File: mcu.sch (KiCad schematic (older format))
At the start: 16 parts, among them SW1 SW_PUSH, U1 STM32F411RE_LQFP64, X1 32.768K, X2 8MHz

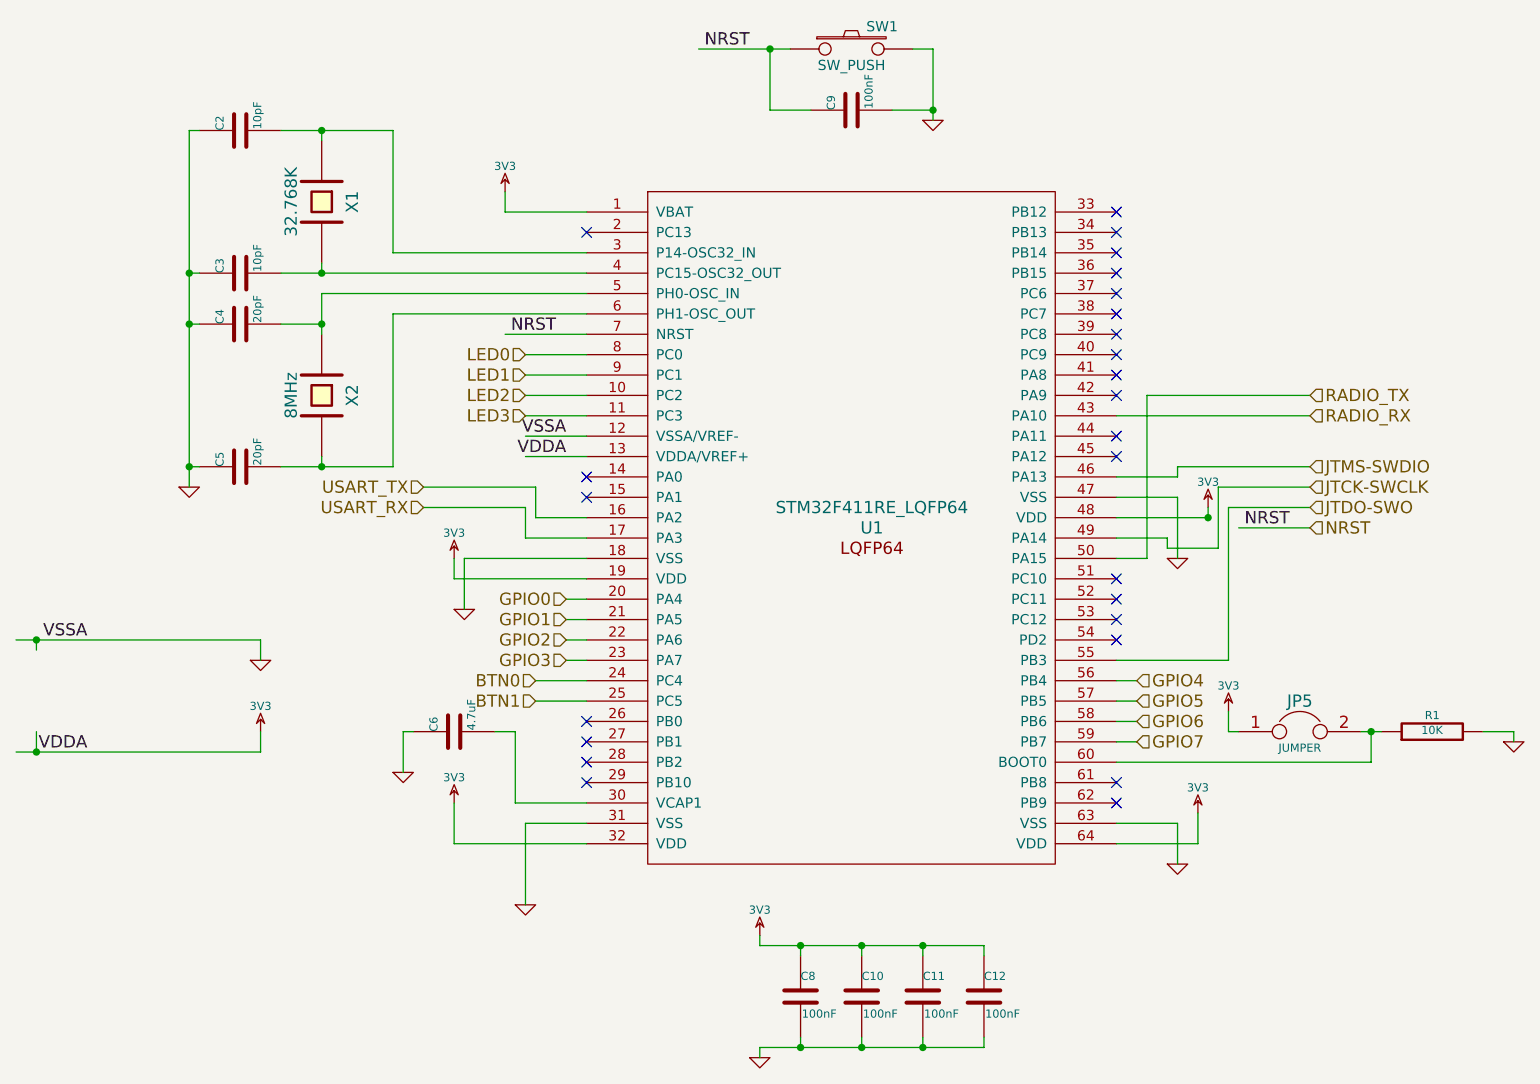
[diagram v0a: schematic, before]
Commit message: Made breakout board
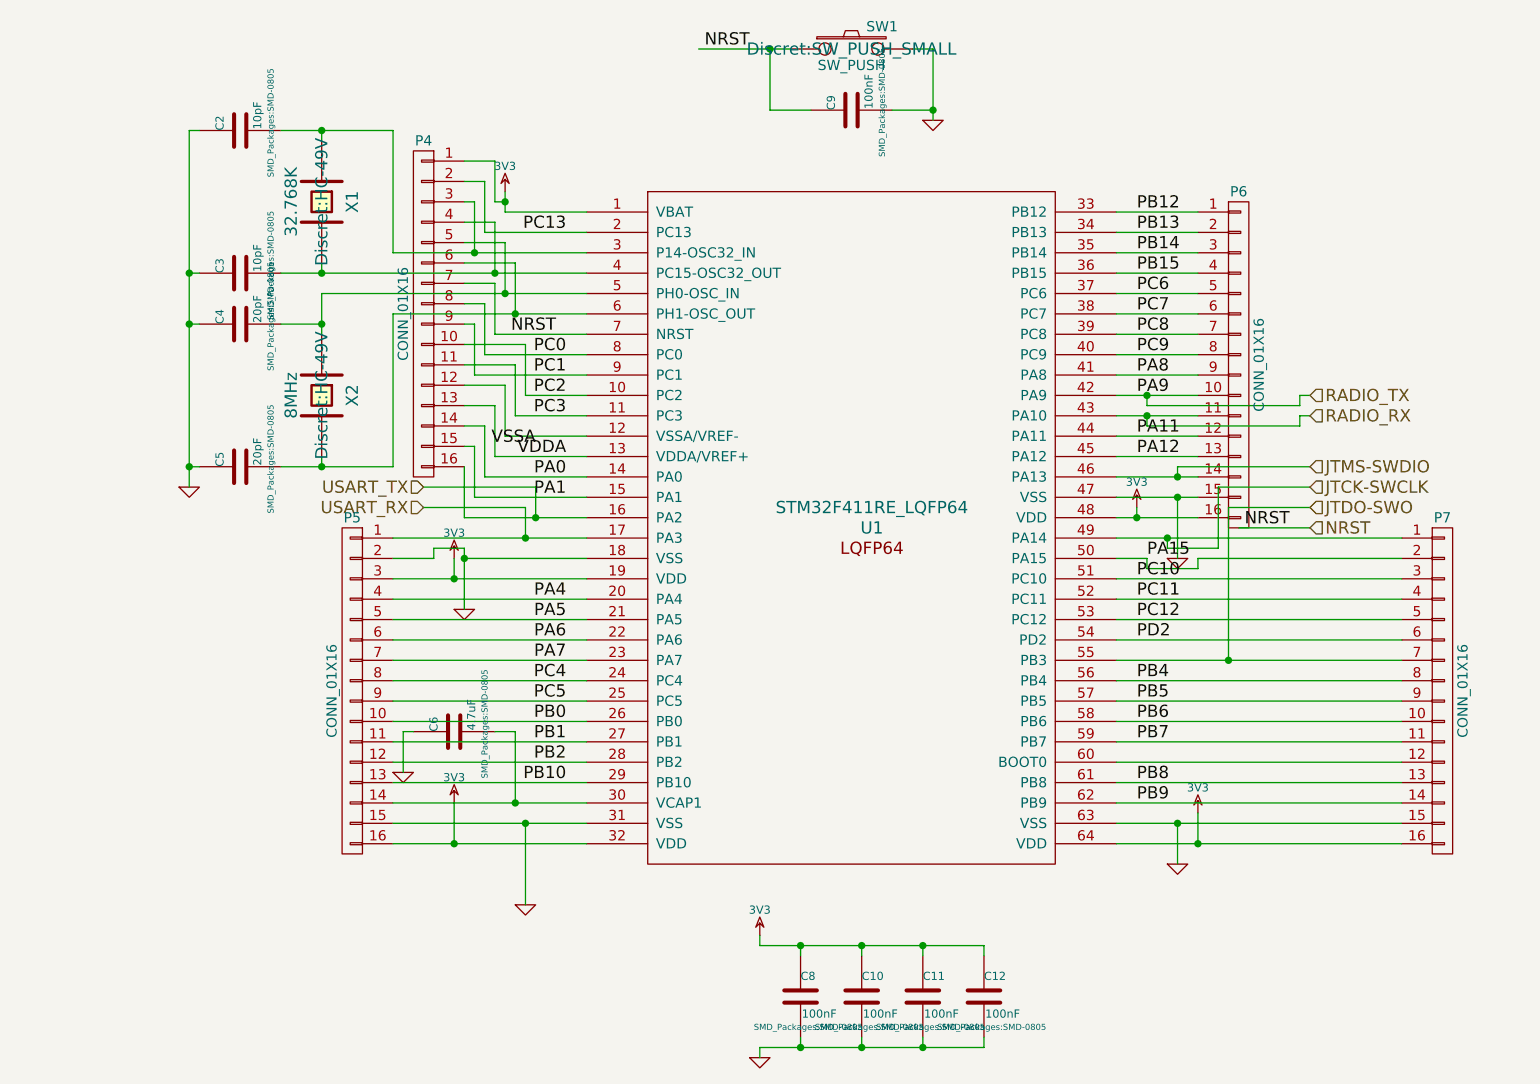
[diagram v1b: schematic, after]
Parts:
- removed JP5: JUMPER, ~, symbol JUMPER
- removed R1: 10K, ~, symbol R
- added P4, P5, P6, P7: CONN_01X16, Pin_Headers:Pin_Header_Straight_1x16, symbol CONN_01X16
- C10, C11, C12, C2, C3, C4, C5, C6, C8, C9: footprint ~ -> SMD_Packages:SMD-0805
- SW1: footprint ~ -> Discret:SW_PUSH_SMALL
- U1: footprint (none) -> Housings_QFP:LQFP-64_10x10mm_Pitch0.5mm
- X1, X2: footprint ~ -> Discret:HC-49V
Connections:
- net labels added: PA0, PA1, PA11, PA12, PA15, PA4, PA5, PA6, PA7, PA8, PA9, PB0, PB1, PB10, PB12, PB13, PB14, PB15, PB2, PB4, PB5, PB6, PB7, PB8, PB9, PC0, PC1, PC10, PC11, PC12, PC13, PC2, PC3, PC4, PC5, PC6, PC7, PC8, PC9, PD2
- net labels removed: BTN0, BTN1, GPIO0, GPIO1, GPIO2, GPIO3, GPIO4, GPIO5, GPIO6, GPIO7, LED0, LED1, LED2, LED3
- wire segments 111 -> 169
- no-connect marks 25 -> 0
